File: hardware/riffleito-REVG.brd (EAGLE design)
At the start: 74.8 x 18 mm, 31 parts, among them IC1 ATMEGA328P, IC2 24AA128SN, IC4 MCP1700-33, X1 16 MHz

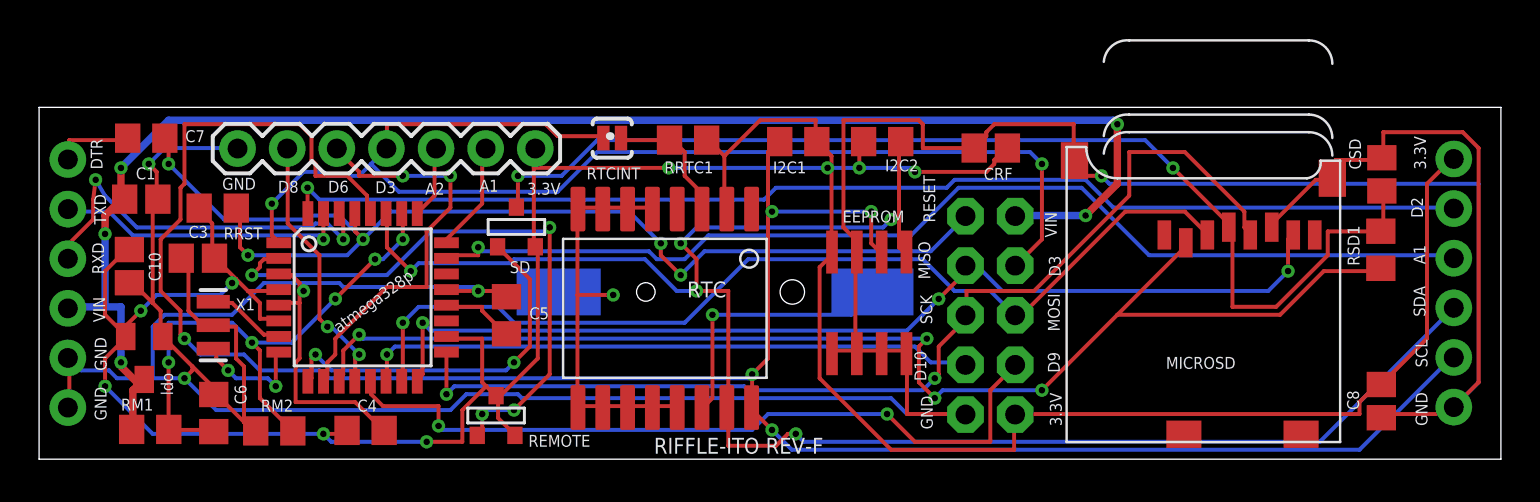
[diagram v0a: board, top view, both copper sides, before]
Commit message: update
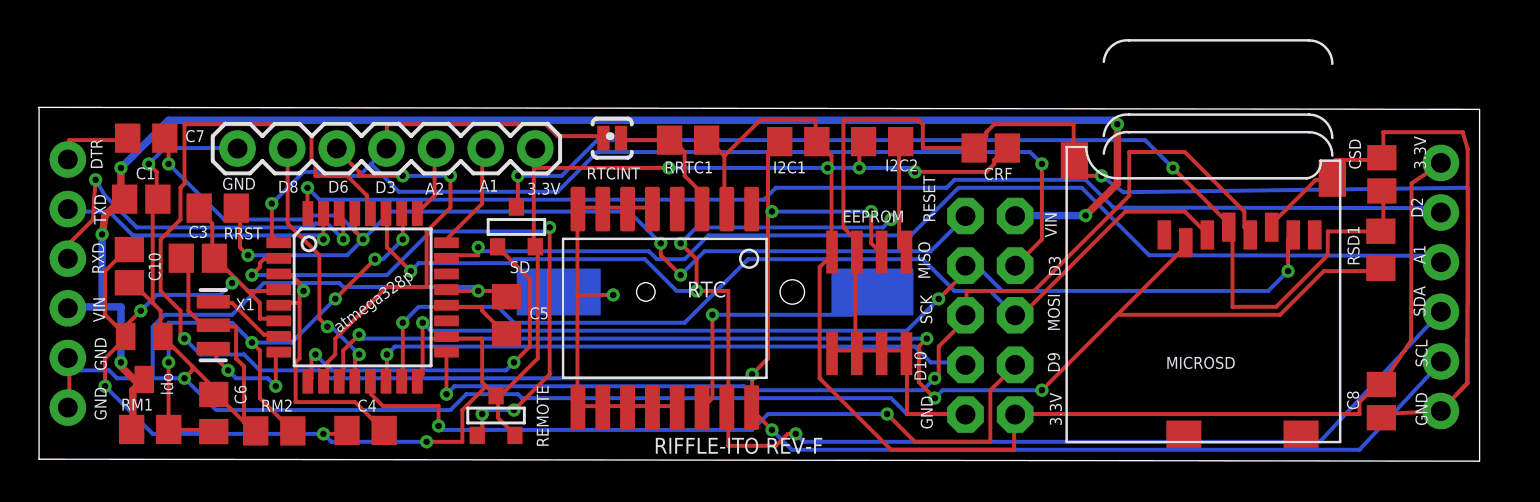
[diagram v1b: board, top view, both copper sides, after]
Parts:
- moved SENSE 0.69 mm to (71.8, 2.39)
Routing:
- net GND: track 255.9 -> 254.6 mm
- net A0: track 55.4 -> 54.7 mm
- net D2: track 61.3 -> 60.6 mm
- net SCL: track 115.6 -> 115.0 mm
- net SDA: track 89.4 -> 88.8 mm
- net VCC: track 167.0 -> 166.5 mm
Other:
- board size 74.8 x 18 mm -> 73.7 x 18.1 mm
